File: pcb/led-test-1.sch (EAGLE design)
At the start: 2 parts

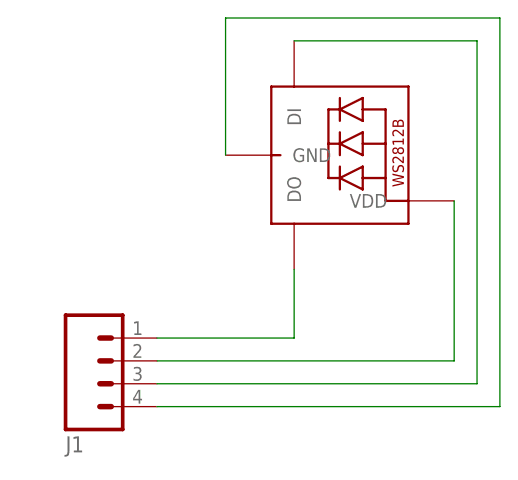
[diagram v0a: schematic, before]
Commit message: added led-test v2
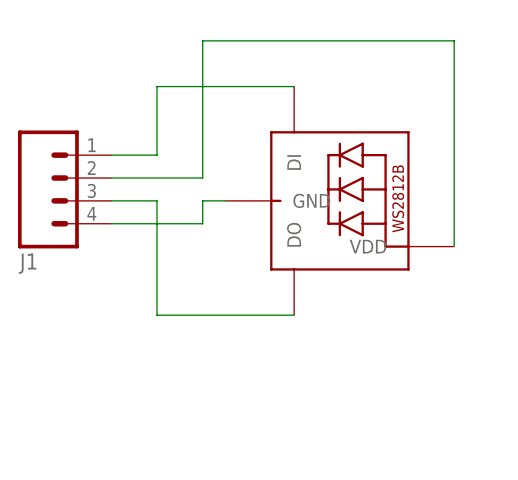
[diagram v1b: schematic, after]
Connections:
- removed net N$2 (its old number): J1.1, LED-2.DO
- removed net N$4 (its old number): J1.3, LED-2.DI
- new net N$1: J1.1, LED-2.DI
- new net N$3: J1.3, LED-2.DO
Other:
- moved on the sheet: J1
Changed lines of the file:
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@@
 </plain>
 <instances>
-<instance part="LED-2" gate="G$1" x="66.04" y="223.52" rot="R270"/>
-<instance part="J1" gate="G$1" x="43.18" y="200.66" rot="MR180"/>
+<instance part="LED-2" gate="G$1" x="66.04" y="218.44" rot="R270"/>
+<instance part="J1" gate="G$1" x="38.1" y="220.98" rot="MR180"/>
 </instances>
 <busses>
@@
 <net name="N$1" class="0">
 <segment>
-<pinref part="LED-2" gate="G$1" pin="GND"/>
-<pinref part="J1" gate="G$1" pin="4"/>
-<wire x1="48.26" y1="195.58" x2="86.36" y2="195.58" width="0.1524" layer="91"/>
-<wire x1="86.36" y1="195.58" x2="86.36" y2="238.76" width="0.1524" layer="91"/>
-<wire x1="86.36" y1="238.76" x2="55.88" y2="238.76" width="0.1524" layer="91"/>
-<wire x1="55.88" y1="238.76" x2="55.88" y2="223.52" width="0.1524" layer="91"/>
+<pinref part="J1" gate="G$1" pin="1"/>
+<pinref part="LED-2" gate="G$1" pin="DI"/>
+<wire x1="43.18" y1="223.52" x2="48.26" y2="223.52" width="0.1524" layer="91"/>
+<wire x1="48.26" y1="223.52" x2="48.26" y2="231.14" width="0.1524" layer="91"/>
+<wire x1="48.26" y1="231.14" x2="63.5" y2="231.14" width="0.1524" layer="91"/>
 </segment>
 </net>
 <net name="N$2" class="0">
 <segment>
-<pinref part="LED-2" gate="G$1" pin="DO"/>
-<wire x1="63.5" y1="210.82" x2="63.5" y2="203.2" width="0.1524" layer="91"/>
-<pinref part="J1" gate="G$1" pin="1"/>
-<wire x1="48.26" y1="203.2" x2="63.5" y2="203.2" width="0.1524" layer="91"/>
+<pinref part="J1" gate="G$1" pin="2"/>
+<wire x1="43.18" y1="220.98" x2="53.34" y2="220.98" width="0.1524" layer="91"/>
+<wire x1="53.34" y1="220.98" x2="53.34" y2="236.22" width="0.1524" layer="91"/>
+<pinref part="LED-2" gate="G$1" pin="VDD"/>
+<wire x1="53.34" y1="236.22" x2="81.28" y2="236.22" width="0.1524" layer="91"/>
+<wire x1="81.28" y1="236.22" x2="81.28" y2="213.36" width="0.1524" layer="91"/>
 </segment>
 </net>
 <net name="N$3" class="0">
 <segment>
-<pinref part="LED-2" gate="G$1" pin="VDD"/>
-<wire x1="81.28" y1="200.66" x2="81.28" y2="218.44" width="0.1524" layer="91"/>
-<pinref part="J1" gate="G$1" pin="2"/>
-<wire x1="48.26" y1="200.66" x2="81.28" y2="200.66" width="0.1524" layer="91"/>
+<pinref part="LED-2" gate="G$1" pin="DO"/>
+<wire x1="63.5" y1="205.74" x2="48.26" y2="205.74" width="0.1524" layer="91"/>
+<wire x1="48.26" y1="205.74" x2="48.26" y2="218.44" width="0.1524" layer="91"/>
+<pinref part="J1" gate="G$1" pin="3"/>
+<wire x1="48.26" y1="218.44" x2="43.18" y2="218.44" width="0.1524" layer="91"/>
 </segment>
 </net>
 <net name="N$4" class="0">
 <segment>
-<pinref part="LED-2" gate="G$1" pin="DI"/>
-<wire x1="63.5" y1="236.22" x2="83.82" y2="236.22" width="0.1524" layer="91"/>
-<wire x1="83.82" y1="236.22" x2="83.82" y2="198.12" width="0.1524" layer="91"/>
-<pinref part="J1" gate="G$1" pin="3"/>
-<wire x1="83.82" y1="198.12" x2="48.26" y2="198.12" width="0.1524" layer="91"/>
+<pinref part="J1" gate="G$1" pin="4"/>
+<wire x1="43.18" y1="215.9" x2="53.34" y2="215.9" width="0.1524" layer="91"/>
+<wire x1="53.34" y1="215.9" x2="53.34" y2="218.44" width="0.1524" layer="91"/>
+<pinref part="LED-2" gate="G$1" pin="GND"/>
+<wire x1="53.34" y1="218.44" x2="55.88" y2="218.44" width="0.1524" layer="91"/>
 </segment>
 </net>
